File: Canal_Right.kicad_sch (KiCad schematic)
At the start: 0 parts

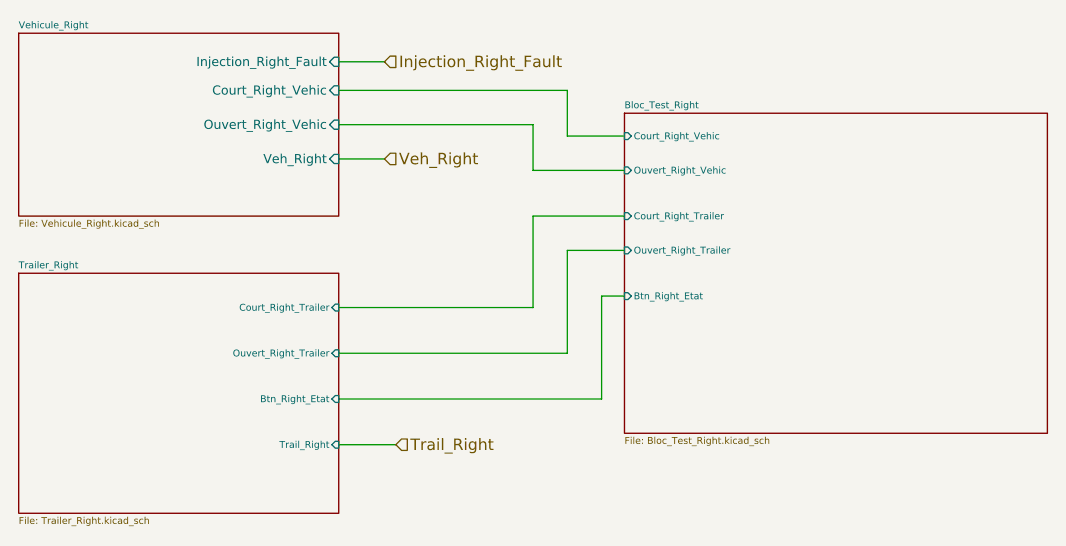
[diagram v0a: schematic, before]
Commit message: Add files via upload
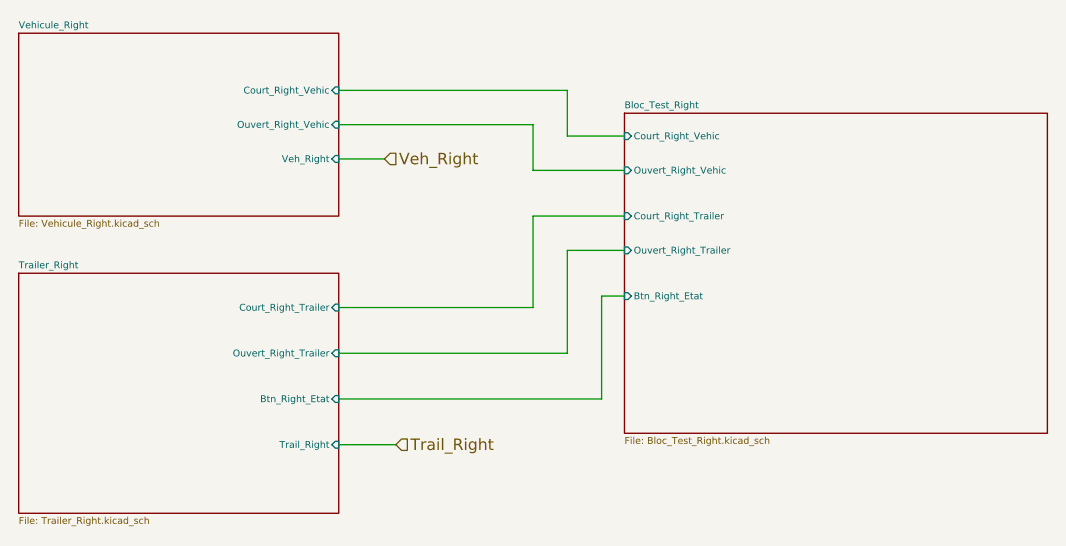
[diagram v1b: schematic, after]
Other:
- sheet Vehicule_Right ports: added none; removed Injection_Right_Fault
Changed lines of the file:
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@@
-	(wire
-		(pts
-			(xy 63.5 33.655) (xy 68.58 33.655)
-		)
-		(stroke
-			(width 0)
-			(type default)
-		)
-	)
 	(wire
 		(pts
@@
 			(width 0)
 			(type default)
-		)
-	)
-	(hierarchical_label "Injection_Right_Fault"
-		(shape input)
-		(at 68.58 33.655 0)
-		(effects
-			(font
-				(size 1.27 1.27)
-			)
-			(justify left)
 		)
 	)
@@
 			(effects
 				(font
-					(size 1.016 1.016)
+					(size 0.762 0.762)
 				)
 				(justify right)
@@
 			(effects
 				(font
-					(size 1.016 1.016)
+					(size 0.762 0.762)
 				)
 				(justify right)
@@
 			(effects
 				(font
-					(size 1.016 1.016)
-				)
-				(justify right)
-			)
-		)
-		(pin "Injection_Right_Fault" input
-			(at 63.5 33.655 0)
-			(effects
-				(font
-					(size 1.016 1.016)
-				)
-				(justify right)
+					(size 0.762 0.762)
+				)
+				(justify right)

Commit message: Add files via upload
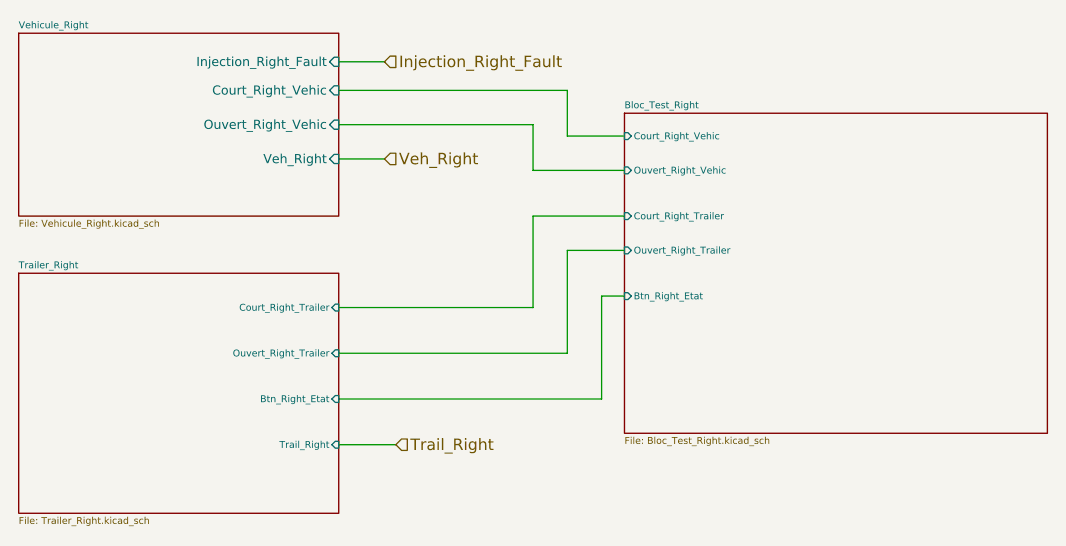
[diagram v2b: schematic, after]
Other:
- sheet Vehicule_Right ports: added Injection_Right_Fault; removed none
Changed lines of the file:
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@@
+	(wire
+		(pts
+			(xy 63.5 33.655) (xy 68.58 33.655)
+		)
+		(stroke
+			(width 0)
+			(type default)
+		)
+	)
 	(wire
 		(pts
@@
 			(width 0)
 			(type default)
+		)
+	)
+	(hierarchical_label "Injection_Right_Fault"
+		(shape input)
+		(at 68.58 33.655 0)
+		(effects
+			(font
+				(size 1.27 1.27)
+			)
+			(justify left)
 		)
 	)
@@
 			(effects
 				(font
-					(size 0.762 0.762)
+					(size 1.016 1.016)
 				)
 				(justify right)
@@
 			(effects
 				(font
-					(size 0.762 0.762)
+					(size 1.016 1.016)
 				)
 				(justify right)
@@
 			(effects
 				(font
-					(size 0.762 0.762)
-				)
-				(justify right)
+					(size 1.016 1.016)
+				)
+				(justify right)
+			)
+		)
+		(pin "Injection_Right_Fault" input
+			(at 63.5 33.655 0)
+			(effects
+				(font
+					(size 1.016 1.016)
+				)
+				(justify right)
